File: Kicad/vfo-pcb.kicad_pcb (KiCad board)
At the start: 2 copper layers, 108.3 x 82.9 mm, 81 parts, among them J1 Rotery Encoder1, J10 Link-out 1-0, J11 Link-out 1-1, J12 Link-out 1-2, J13 Link-out 2-0, J14 Link-out 2-1, J15 Link-out 2-2, J2 Rotery Encoder2, J3 Analog in 3-6, J4 RxTx, J5 V12, J6 ESP32L, J7 ESP32R, J8 ILI9341, J9 Conn_01x07_Female, Q1 BFR92, Q2 BFR92, Q3 BFR92, Q4 BFR92, Q5 BFR92, Q6 BFR92, SW1 Rotary_Encoder_Switch, U1 L7805, U2 Si5351A-B-GT, U3 Si5351A-B-GT, U4 AMS1117, Y1 Crystal, Y2 Crystal

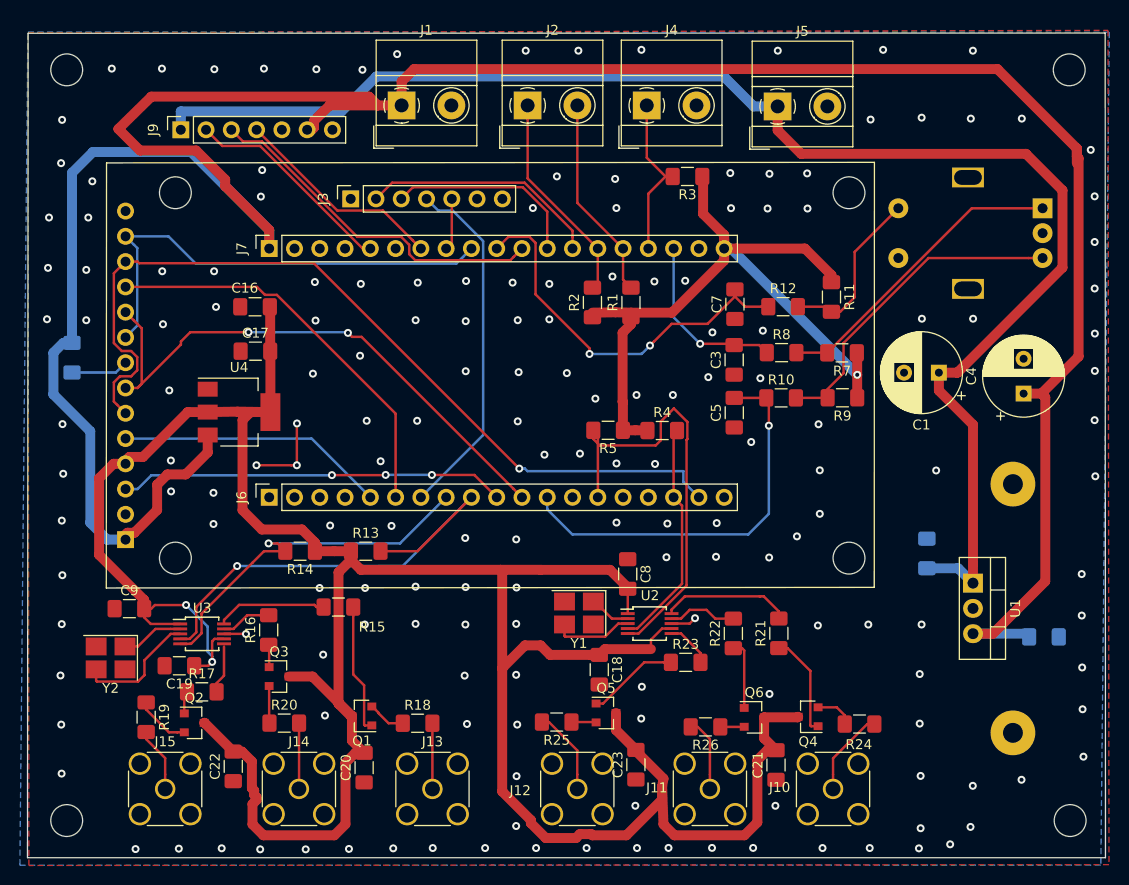
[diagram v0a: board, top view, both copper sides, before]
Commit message: Add files via upload
Updated output circuit added pi attenuation
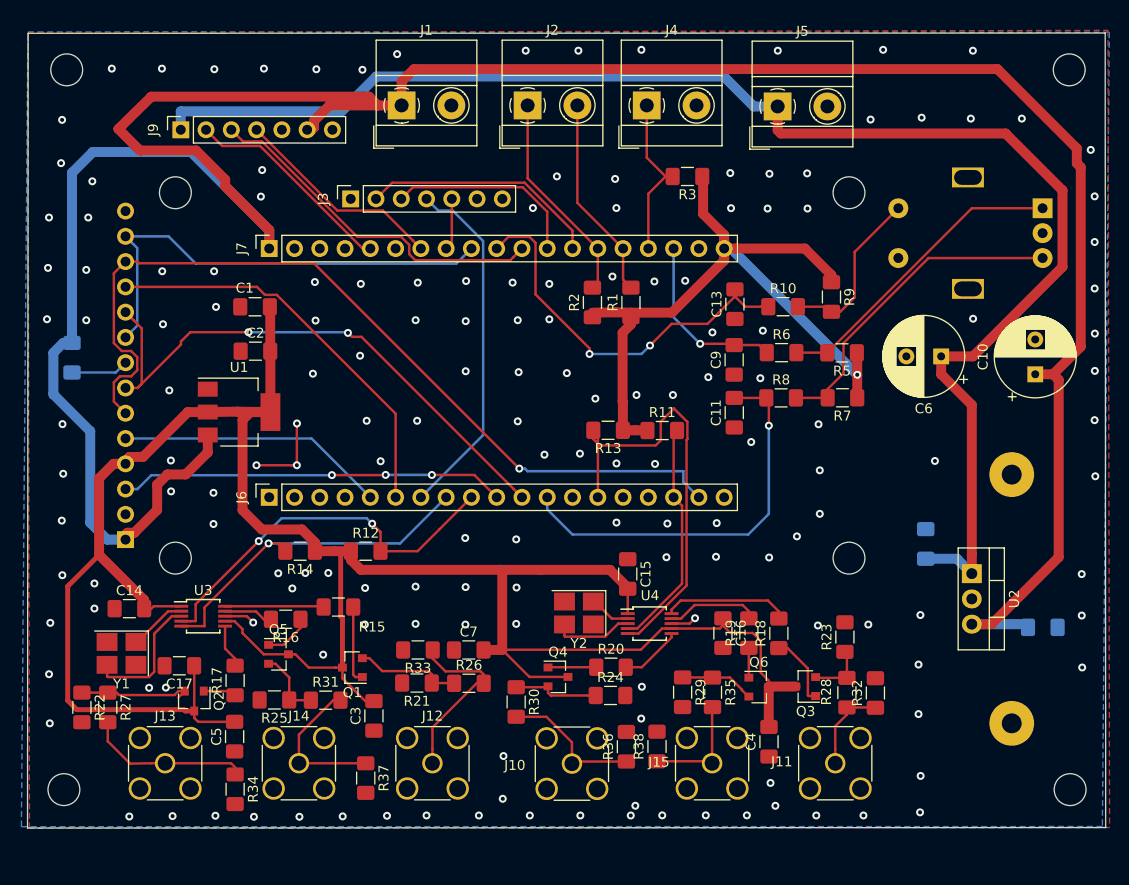
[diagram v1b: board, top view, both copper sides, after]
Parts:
- added R19: 1k, Resistor_SMD:R_1206_3216Metric_Pad1.42x1.75mm_HandSolder, F.Cu at (114.8, 112.6)
- added R21: 150, Resistor_SMD:R_1206_3216Metric_Pad1.42x1.75mm_HandSolder, F.Cu at (81.5, 117.7)
- added R23: 150, Resistor_SMD:R_1206_3216Metric_Pad1.42x1.75mm_HandSolder, F.Cu at (124.5, 113.0)
- added R24: 150, Resistor_SMD:R_1206_3216Metric_Pad1.42x1.75mm_HandSolder, F.Cu at (100.9, 118.9)
- added R25: 150, Resistor_SMD:R_1206_3216Metric_Pad1.42x1.75mm_HandSolder, F.Cu at (67.1, 119.3)
- added R29: 150, Resistor_SMD:R_1206_3216Metric_Pad1.42x1.75mm_HandSolder, F.Cu at (108.2, 118.6)
- added R32: 150, Resistor_SMD:R_1206_3216Metric_Pad1.42x1.75mm_HandSolder, F.Cu at (127.5, 118.7)
- added R33: 150, Resistor_SMD:R_1206_3216Metric_Pad1.42x1.75mm_HandSolder, F.Cu at (81.5, 114.3)
- added R34: 150, Resistor_SMD:R_1206_3216Metric_Pad1.42x1.75mm_HandSolder, F.Cu at (63.2, 128.3)
- added R36: 150, Resistor_SMD:R_1206_3216Metric_Pad1.42x1.75mm_HandSolder, F.Cu at (102.5, 124.0)
- added R37: 150, Resistor_SMD:R_1206_3216Metric_Pad1.42x1.75mm_HandSolder, F.Cu at (76.3, 127.2)
- added R38: 150, Resistor_SMD:R_1206_3216Metric_Pad1.42x1.75mm_HandSolder, F.Cu at (105.6, 124.0)
- R22: value 1k -> 150
- R26: renamed from R18; value 20 -> 33
- R27: renamed from R19; value 20 -> 33
- R28: renamed from R24; value 20 -> 33
- R30: renamed from R25; value 20 -> 33
- R31: renamed from R20; value 20 -> 33
- R35: renamed from R26; value 47 -> 33
- moved R22 65.9 mm to (47.8, 120.1), turned to 270 degrees
- moved C7 20.4 mm to (86.7, 114.3), turned to 0 degrees
- moved C16 13.0 mm to (112.2, 112.6)
- moved R20 7.52 mm to (100.9, 116.1)
- moved R26 6.54 mm to (86.7, 117.7)
- moved Q4 6.04 mm to (95.6, 117.0)
- moved C3 5.29 mm to (77.1, 121.0)
- moved Q1 4.95 mm to (75.0, 116.1)
- moved R31 4.76 mm to (72.3, 119.4)
- moved R30 4.54 mm to (91.4, 119.6), turned to 270 degrees
- moved R27 3.98 mm to (50.4, 120.1)
- moved R35 3.54 mm to (111.2, 118.6), turned to 270 degrees
- moved R17 3.54 mm to (63.2, 117.4), turned to 90 degrees
- moved R28 3.40 mm to (124.7, 118.6), turned to 270 degrees
- moved   3.12 mm to (46.0, 128.4)
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- renumbered C16 to C1, C4 to C10, C5 to C11, C6 to C12, C7 to C13, C9 to C14, C8 to C15, C18 to C16, C19 to C17, C17 to C2, C20 to C3, C21 to C4, C22 to C5, C1 to C6, C23 to C7, C2 to C8, C3 to C9, J12 to J10, J10 to J11, J13 to J12, J15 to J13, J11 to J15, Q4 to Q3, Q5 to Q4, Q3 to Q5, R12 to R10, R4 to R11, R13 to R12, R5 to R13, R21 to R18, R23 to R20, R6 to R4, R7 to R5, R8 to R6, R9 to R7, R10 to R8, R11 to R9, U4 to U1, U1 to U2, U2 to U4, Y2 to Y1, Y1 to Y2
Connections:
- R22 pad 1: Net-(Q6-Pad1) -> Net-(Q2-Pad2)
- R22 pad 2: Net-(R22-Pad2) -> GND
- U4 pad 9: Net-(R22-Pad2) -> Net-(R19-Pad2)
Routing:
- net V33a: track 288.5 -> 235.5 mm, vias 2 -> 0
- net Net-(J12-Pad1): track 6.60 -> 18.2 mm
- net Net-(J13-Pad1): track 6.51 -> 16.6 mm
- net Net-(R19-Pad2): track 0.00 -> 9.31 mm
- net SCL_2: track 48.0 -> 39.2 mm, vias 1 -> 2
- net Net-(J14-Pad1): track 6.62 -> 15.2 mm
- net Net-(Q1-Pad2): track 3.84 -> 10.8 mm
- net Net-(R22-Pad2): track 6.94 -> 0.00 mm
- net Net-(Q4-Pad2): track 2.49 -> 8.79 mm
- net Net-(Q2-Pad2): track 5.49 -> 11.5 mm
- net Net-(J10-Pad1): track 8.61 -> 14.4 mm
- net Net-(Q1-Pad1): track 13.1 -> 7.83 mm
- net Net-(Q6-Pad2): track 2.41 -> 7.48 mm
- net Net-(Q4-Pad1): track 9.23 -> 4.85 mm
- net Net-(Q6-Pad1): track 6.96 -> 2.99 mm
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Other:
- board size 108.3 x 82.9 mm -> 108.4 x 79.9 mm
- net class power: clearance 0.5 -> 0.3; trace_width 1 -> 0.5
